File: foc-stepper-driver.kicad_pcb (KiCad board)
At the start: 4 copper layers, 42 x 42 mm, 72 parts, among them CN1 C42391660, CN2 C2839706, CN3 C2839705, CN4 C2839704, J2 TC2030, U1 DRV8962DDWR, U2 TYPE-C 16PLT-H10.0, U3 STM32G431CBT6, U6 AS5047P-ATSM, U7 TPS560430XDBVR, U8 SPX3819M5-L-3-3/TR, U9 TCAN3403DRQ1, X1 NX3215SA 32.768KHZ EXS00A-MU0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, X2 NDK NX2016SA-24MHZ-EXS00A-CS1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

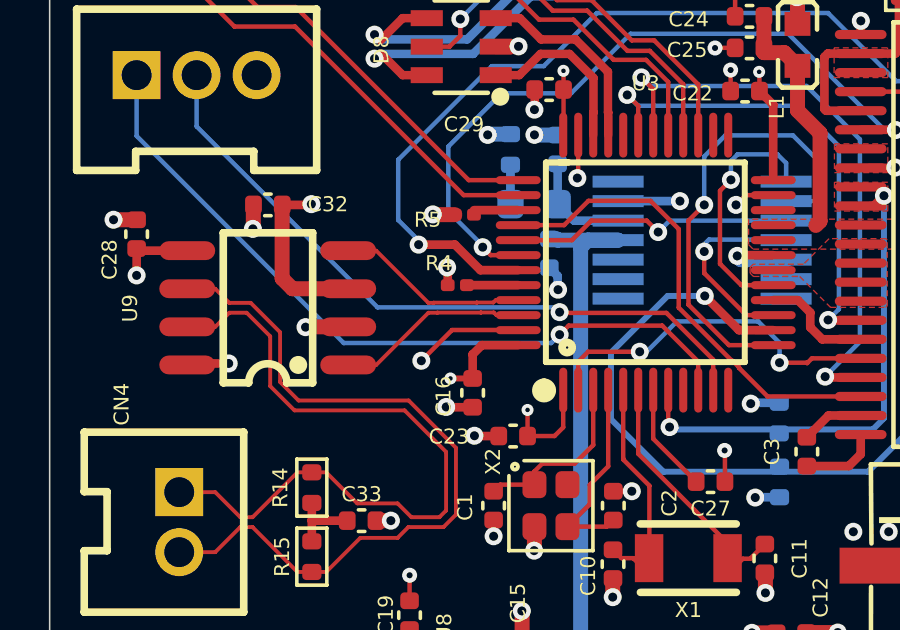
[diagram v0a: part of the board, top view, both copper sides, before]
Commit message: update
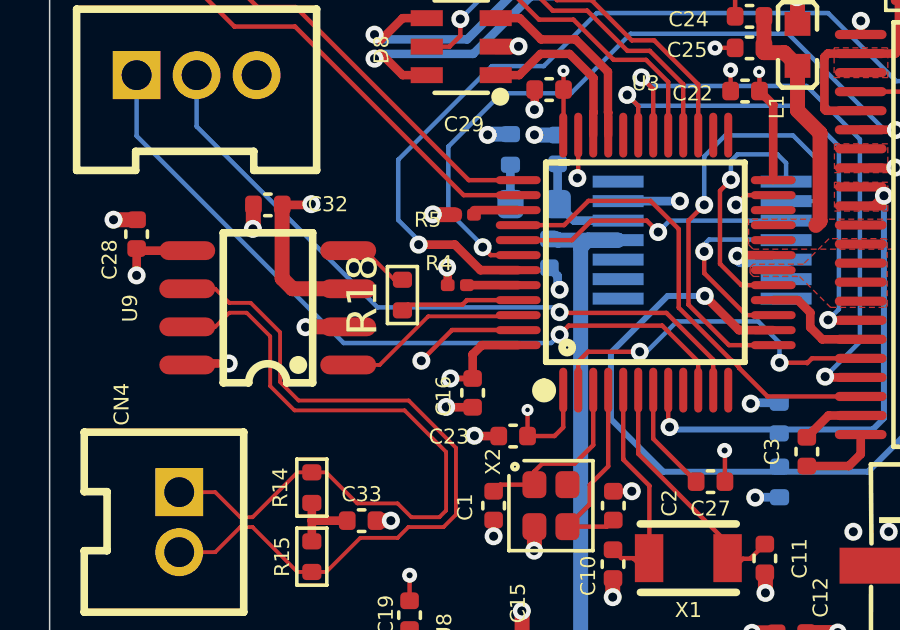
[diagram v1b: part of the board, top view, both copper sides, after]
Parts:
- added R18: 1k, PCM_Resistor_SMD_AKL:R_0402_1005Metric, F.Cu at (126.1, 85.6)
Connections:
- net /STM32G431CBT6/STM32_CANFD- renamed /STM32G431CBT6/STM32_CANFD_TX
- U3 pad 45: /STM32G431CBT6/STM32_CANFD+ -> Net-(U3-PB8-BOOT0)
- U9 pad 4: /STM32G431CBT6/STM32_CANFD+ -> /STM32G431CBT6/STM32_CANFD_RX
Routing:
- net /STM32G431CBT6/STM32_CANFD+: track 6.43 -> 0.00 mm
- net Net-(U3-PB8-BOOT0): track 0.00 -> 4.01 mm
- net /STM32G431CBT6/STM32_CANFD_RX: track 0.00 -> 2.20 mm

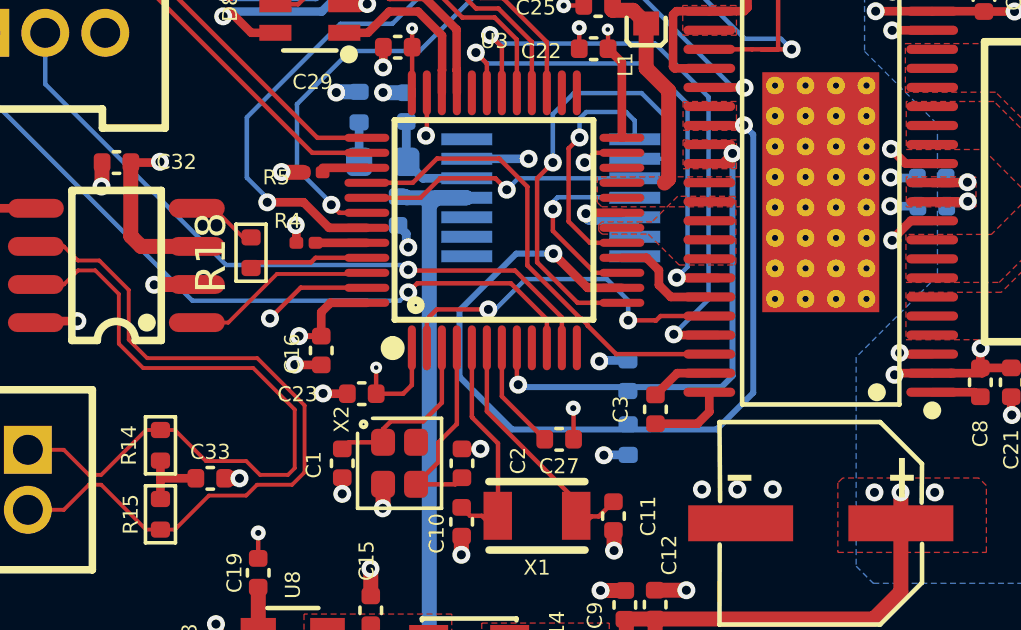
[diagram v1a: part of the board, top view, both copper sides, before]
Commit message: update
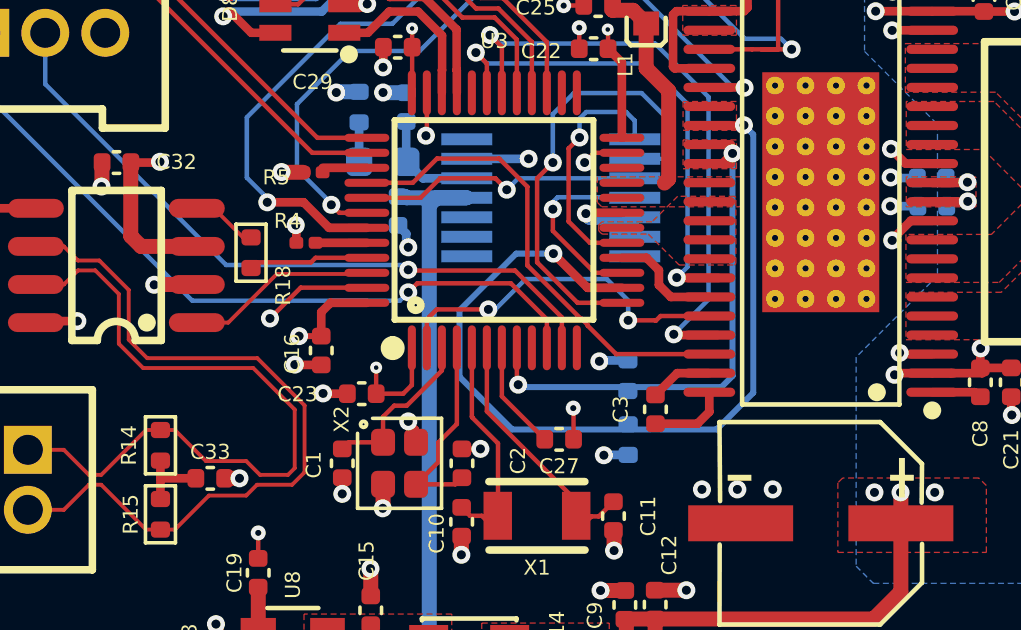
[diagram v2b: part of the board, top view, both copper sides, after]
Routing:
- net GND: track 63.4 -> 63.6 mm, vias 59 -> 60
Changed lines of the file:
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@@
 		(tags "resistor")
 		(property "Reference" "R18"
-			(at 0 -1.3335 90)
+			(at -1.09 1.07 90)
 			(layer "F.SilkS")
 			(effects
 				(font
-					(size 1 1)
-					(thickness 0.15)
+					(size 0.5 0.5)
+					(thickness 0.125)
 				)
 			)
@@
 	)
 	(segment
+		(start 131.56 91.462614)
+		(end 131.3 91.202614)
+		(width 0.2)
+		(layer "F.Cu")
+		(net 1)
+	)
+	(segment
 		(start 136.81 90.77)
 		(end 136.8 90.76)
@@
 	)
 	(segment
+		(start 131.56 91.9)
+		(end 131.56 91.462614)
+		(width 0.2)
+		(layer "F.Cu")
+		(net 1)
+	)
+	(segment
 		(start 136.61 70.46)
 		(end 136.61 71.26)
@@
 	)
 	(segment
-		(start 145.465553 83.978553)
-		(end 145.05 83.563)
-		(width 0.5)
-		(layer "F.Cu")
-		(net 1)
-	)
-	(segment
 		(start 120.269966 87.860034)
 		(end 120.27 87.86)
@@
 	)
 	(via
+		(at 131.3 91.202614)
+		(size 0.6)
+		(drill 0.3)
+		(layers "F.Cu" "B.Cu")
+		(net 1)
+	)
+	(via
 		(at 130.46 79.4)
 		(size 0.6)
@@
 	)
 	(segment
-		(start 131.8 91.2)
-		(end 130.72 91.2)
+		(start 130.46 91.9)
+		(end 130.46 91.05)
 		(width 0.15)
 		(layer "F.Cu")
@@
 	)
 	(segment
-		(start 130.46 91.46)
-		(end 130.46 91.9)
+		(start 130.46 91.05)
+		(end 130.83 90.68)
 		(width 0.15)
 		(layer "F.Cu")
@@
 	)
 	(segment
-		(start 132.42 88.75)
-		(end 132.42 90.58)
+		(start 131.25 90.68)
+		(end 132.42 89.51)
 		(width 0.15)
 		(layer "F.Cu")
@@
 	)
 	(segment
-		(start 132.42 90.58)
-		(end 131.8 91.2)
+		(start 132.42 89.51)
+		(end 132.42 88.75)
 		(width 0.15)
 		(layer "F.Cu")
@@
 	)
 	(segment
-		(start 130.72 91.2)
-		(end 130.46 91.46)
+		(start 130.46 91.9)
+		(end 129.32 91.9)
 		(width 0.15)
 		(layer "F.Cu")
@@
 	)
 	(segment
-		(start 130.46 91.9)
-		(end 129.32 91.9)
+		(start 130.83 90.68)
+		(end 131.25 90.68)
 		(width 0.15)
 		(layer "F.Cu")
